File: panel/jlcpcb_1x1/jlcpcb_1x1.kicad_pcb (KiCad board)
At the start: 4 copper layers, 70.5 x 70.5 mm, 185 parts, among them U108 Single Buffer - 74LVC1G125GV,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, U109 3.3v LDO - TLV74133PDBVR

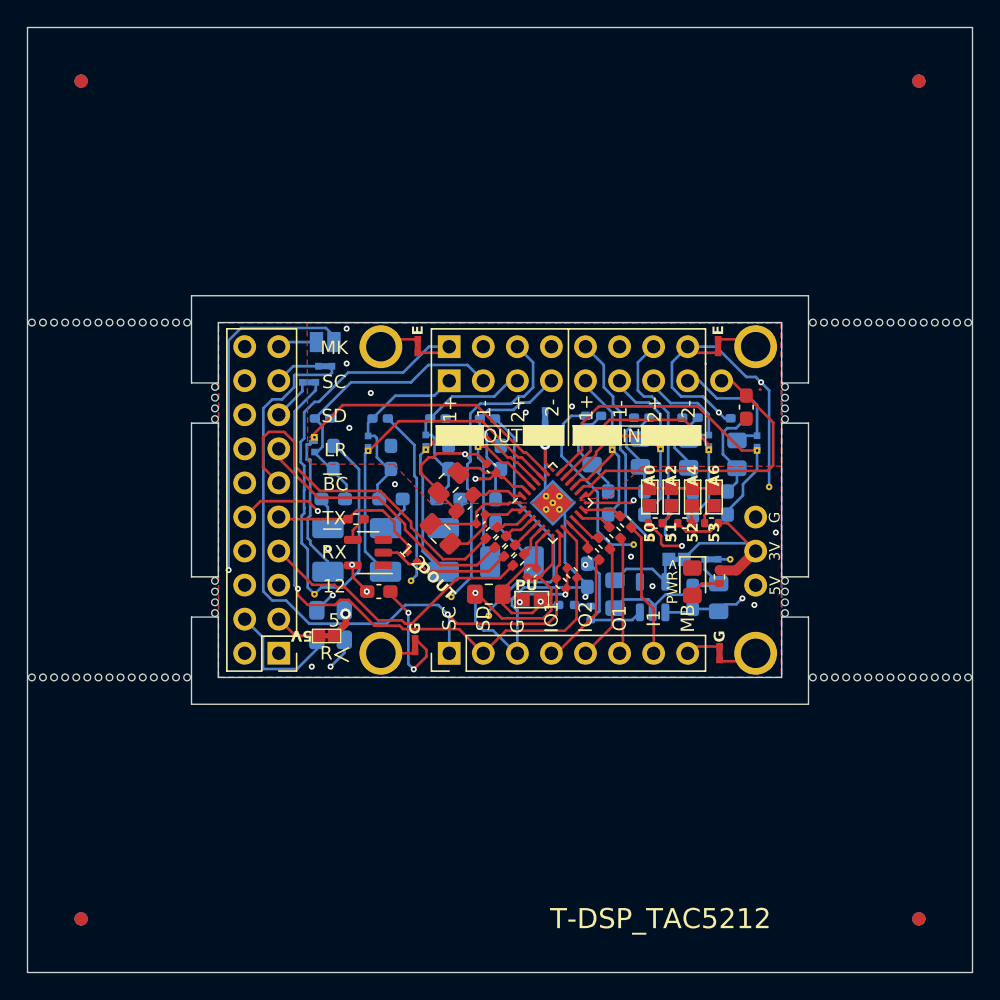
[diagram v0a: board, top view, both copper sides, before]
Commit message: update
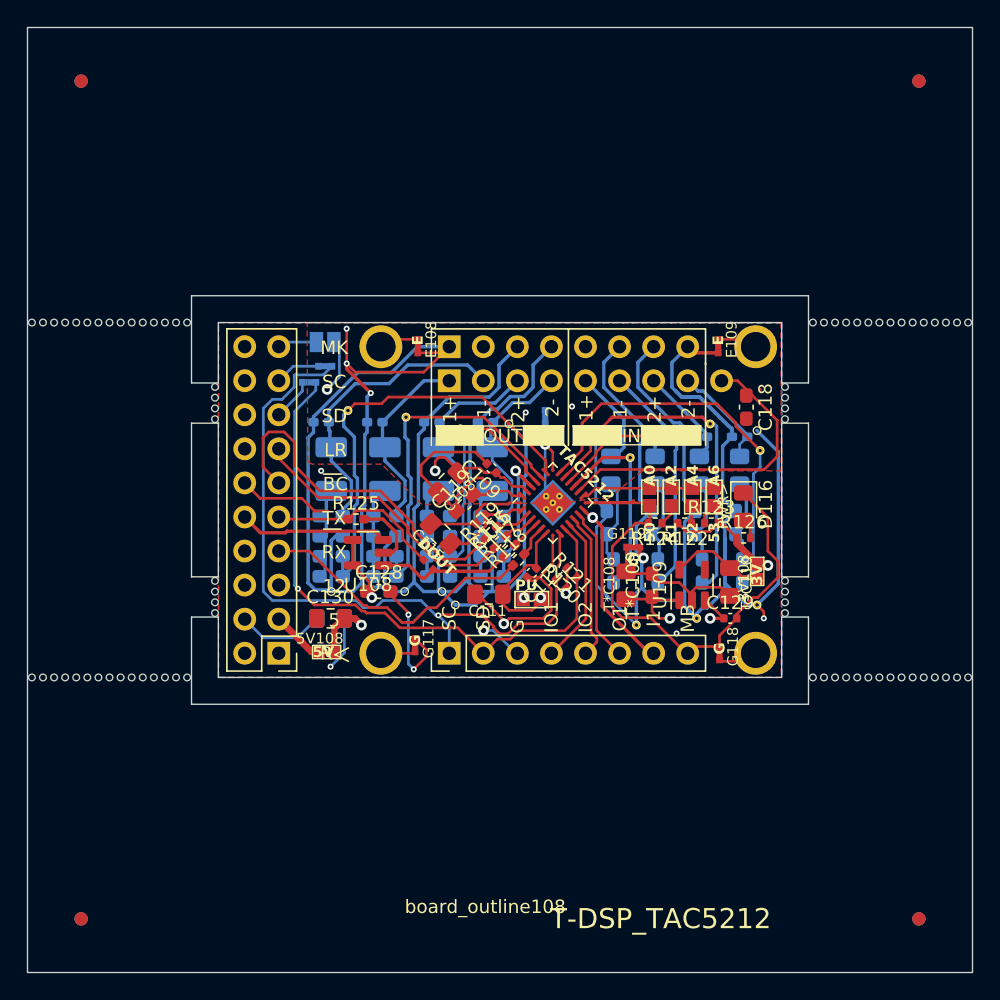
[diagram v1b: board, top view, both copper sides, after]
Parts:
- removed G115: VIA, project_fp:via
- removed OM1: Jump Filter, project_fp:jumper_slice_via_alt_text
- removed OM2, OP1, OP2: Jump Filter, project_fp:jumper_slice_via
- removed R110, R112, R113, R114: 0 Ohm, project_fp:R_0402_1005Metric_Pad0.72x0.64mm_HandSolder
- removed R128: 2.21k ohm, project_fp:R_0402_1005Metric
- removed SCL109: jumper, Resistor_SMD:R_0402_1005Metric_Pad0.72x0.64mm_HandSolder
- added G123: SMD ROUTING PAD, project_fp:SMD_ROUTING_PAD, B.Cu at (149.2, 49.6)
- added OUTM1: VIA, project_fp:via, B.Cu at (137.2, 48.6)
- added OUTP1: VIA, project_fp:via, B.Cu at (141.5, 49.1)
- added OUTP2: VIA, project_fp:via, B.Cu at (145.5, 49.9)
- added R127: DNP, Capacitor_SMD:C_0603_1608Metric_Pad1.08x0.95mm_HandSolder, B.Cu at (139.9, 59.4)
- added R129: 0 ohm, Capacitor_SMD:C_0603_1608Metric_Pad1.08x0.95mm_HandSolder, B.Cu at (139.9, 56.4)
- added R130: 100K, Capacitor_SMD:C_0603_1608Metric_Pad1.08x0.95mm_HandSolder, B.Cu at (166.1, 56.9)
- added R131: DNP, Capacitor_SMD:C_0603_1608Metric_Pad1.08x0.95mm_HandSolder, B.Cu at (143.9, 59.4)
- added R132: 10 ohm, Capacitor_SMD:C_0603_1608Metric_Pad1.08x0.95mm_HandSolder, B.Cu at (143.9, 60.9)
- added R133: 0 ohm, Capacitor_SMD:C_0603_1608Metric_Pad1.08x0.95mm_HandSolder, B.Cu at (143.9, 56.4)
- added R134: DNP, Capacitor_SMD:C_0603_1608Metric_Pad1.08x0.95mm_HandSolder, B.Cu at (147.9, 59.4)
- added R135: 10 ohm, Capacitor_SMD:C_0603_1608Metric_Pad1.08x0.95mm_HandSolder, B.Cu at (147.9, 60.9)
- added R136: 0 ohm, Capacitor_SMD:C_0603_1608Metric_Pad1.08x0.95mm_HandSolder, B.Cu at (147.9, 56.4)
- added R137: 100K, Capacitor_SMD:C_0603_1608Metric_Pad1.08x0.95mm_HandSolder, B.Cu at (163.1, 56.9)
- added R138: 100K, Capacitor_SMD:C_0603_1608Metric_Pad1.08x0.95mm_HandSolder, B.Cu at (159.8, 56.9)
- added R139: 100K, Capacitor_SMD:C_0603_1608Metric_Pad1.08x0.95mm_HandSolder, B.Cu at (156.5, 56.9)
- 3V108, C130, G119, NT108, T*C108, T*C109, T*C110, U109: moved to F.Cu
- C113: value 0.047uF -> 0.0047µF (4.7nF); footprint project_fp:C_0603_1608Metric_Pad1.08x0.95mm_HandSolder -> Capacitor_SMD:C_0603_1608Metric_Pad1.08x0.95mm_HandSolder
- C114, C120, C122: value 47uF -> 0.0047µF (4.7nF); footprint project_fp:CP_EIA-3528-21_Kemet-B_Pad1.50x2.35mm_HandSolder -> Capacitor_SMD:C_0603_1608Metric_Pad1.08x0.95mm_HandSolder
- C117, C121, C123: value 0.047uF -> 47uF; footprint project_fp:C_0603_1608Metric_Pad1.08x0.95mm_HandSolder -> project_fp:CP_EIA-3528-21_Kemet-B_Pad1.50x2.35mm_HandSolder
- C124: value 10UF -> 10UF confirm polarity
- C129: value 1uF -> 0.1uF; footprint project_fp:C_0603_1608Metric_Pad1.08x0.95mm_HandSolder -> project_fp:C_0402_1005Metric; moved to F.Cu
- D108, D109, D110, D111, D112: value TPD1E1B04 - 0402 size -> TPD1E10B06
- G108, G109, G110, G111, G112: footprint project_fp:via -> project_fp:SMD_ROUTING_PAD; moved to B.Cu
- G113, G114, G116: moved to B.Cu
- INM1, INM2, INP1, INP2: value Jump Filter -> VIA; footprint project_fp:jumper_slice_via -> project_fp:via
- R108, R111: value 100 -> 10 ohm; footprint project_fp:R_0603_1608Metric_Pad1.05x0.95mm_HandSolder -> Capacitor_SMD:C_0603_1608Metric_Pad1.08x0.95mm_HandSolder
- R109: value 100 -> DNP; footprint project_fp:R_0603_1608Metric_Pad1.05x0.95mm_HandSolder -> Capacitor_SMD:C_0603_1608Metric_Pad1.08x0.95mm_HandSolder
- R116: value 100 -> 0 ohm; footprint project_fp:R_0603_1608Metric_Pad1.05x0.95mm_HandSolder -> Capacitor_SMD:C_0603_1608Metric_Pad1.08x0.95mm_HandSolder
- R117, R125: value 49.9 ohm -> 27 ohm
- U108: value Single Buffer - 74LVC1G125GV,125 - SOT-23-5 -> Single Buffer with Tri-state Passthru - SN74LVC1G66DCK - SOT-23-5
- board_outline108: footprint project_fp:audio_module_board_outline_50x34.5_d1 -> project_fp:audio_module_board_outline_50x34.5_e1
- moved G112 16.7 mm to (145.2, 63.1), turned to 180 degrees
- moved G110 16.1 mm to (144.2, 62.1), turned to 180 degrees
- moved G113 14.0 mm to (158.7, 64.6), turned to 180 degrees
- moved G108 12.5 mm to (167.7, 50.1), turned to 180 degrees
- moved R116 12.3 mm to (135.9, 56.4), turned to 180 degrees
- moved C129 11.1 mm to (165.7, 64.1), turned to 0 degrees
- moved R111 10.5 mm to (135.9, 60.9)
- moved G116 8.85 mm to (167.7, 63.1), turned to 180 degrees
- moved T*C110 8.62 mm to (165.6, 61.3)
- moved T*C108 6.96 mm to (157.9, 61.6)
- moved D116 6.77 mm to (166.7, 55.6)
- moved G111 6.72 mm to (141.4, 62.1), turned to 180 degrees
- moved 3V108 6.07 mm to (167.7, 60.6), turned to -90 degrees
- moved C110 6.03 mm to (139.9, 52.9)
- moved G109 6.00 mm to (135.9, 62.1), turned to 180 degrees
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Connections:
- C110 pad 1: Board_0-OUT1P -> Board_0-Net-(C110-Pad1)
- C110 pad 2: Board_0-Net-(C110-Pad2) -> Board_0-OUT1P+
- C113 pad 1: Board_0-OUT1P+ -> Board_0-Net-(C110-Pad1)
- C114 pad 1: Board_0-OUT1M -> Board_0-Net-(C114-Pad1)
- C114 pad 2: Board_0-Net-(C114-Pad2) -> Board_0-Earth
- C117 pad 1: Board_0-OUT1M+ -> Board_0-Net-(C114-Pad1)
- C117 pad 2: Board_0-Earth -> Board_0-OUT1M+
- C120 pad 1: Board_0-OUT2P -> Board_0-Net-(C120-Pad1)
- C120 pad 2: Board_0-Net-(C120-Pad2) -> Board_0-Earth
- C121 pad 1: Board_0-OUT2P+ -> Board_0-Net-(C120-Pad1)
- C121 pad 2: Board_0-Earth -> Board_0-OUT2P+
- C122 pad 1: Board_0-OUT2M -> Board_0-Net-(C122-Pad1)
- C122 pad 2: Board_0-Net-(C122-Pad2) -> Board_0-Earth
- C123 pad 1: Board_0-OUT2M+ -> Board_0-Net-(C122-Pad1)
- C123 pad 2: Board_0-Earth -> Board_0-OUT2M+
- D112 pad 1: Board_0-Net-(C124-Pad1) -> Board_0-IN2M+
- D113 pad 1: Board_0-Net-(C125-Pad1) -> Board_0-IN2P+
- D114 pad 1: Board_0-Net-(C126-Pad1) -> Board_0-IN1M+
- D115 pad 1: Board_0-Net-(C127-Pad1) -> Board_0-IN1P+
- INM1 pad 1: Board_0-IN1M+ -> Board_0-IN1M
- INM2 pad 1: Board_0-IN2M+ -> Board_0-IN2M
- INP1 pad 1: Board_0-IN1P+ -> Board_0-IN1P
- INP2 pad 1: Board_0-IN2P+ -> Board_0-IN2P
- R108 pad 1: Board_0-OUT1P+ -> Board_0-Net-(C110-Pad1)
- R108 pad 2: Board_0-Net-(C110-Pad2) -> Board_0-OUT1P
- R109 pad 1: Board_0-OUT1M+ -> Board_0-Net-(C114-Pad1)
- R109 pad 2: Board_0-Net-(C114-Pad2) -> Board_0-OUT1M
- R111 pad 1: Board_0-OUT2P+ -> Board_0-Net-(C114-Pad1)
- R111 pad 2: Board_0-Net-(C120-Pad2) -> Board_0-OUT1M
- R116 pad 1: Board_0-OUT2M+ -> Board_0-OUT1M+
- R116 pad 2: Board_0-Net-(C122-Pad2) -> Board_0-Net-(C114-Pad1)
- R125 pad 2: Board_0-Net-(U108-Y) -> Board_0-Net-(U108-B)
- TAC5212 pad 10: Board_0-Net-(TAC5212-GPIO2) -> Board_0-GPIO2
- TAC5212 pad 11: Board_0-Net-(TAC5212-GPO1) -> Board_0-GPO1
- TAC5212 pad 12: Board_0-Net-(TAC5212-GPI1) -> Board_0-GPI1
- TAC5212 pad 9: Board_0-Net-(TAC5212-GPIO1) -> Board_0-GPIO1
- U108 pad 1: Board_0-GNDD -> Board_0-5212_DOUT1
- U108 pad 2: Board_0-5212_DOUT1 -> Board_0-Net-(U108-B)
- U108 pad 4: Board_0-Net-(U108-Y) -> Board_0-3.3v_IDE
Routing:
- net Board_0-Earth: track 185.5 -> 295.5 mm, vias 11 -> 8
- net Board_0-GPI1: track 71.6 -> 43.5 mm, vias 1 -> 2
- net Board_0-GNDD: track 108.7 -> 135.8 mm, vias 15 -> 7
- net Board_0-IN1M: track 14.1 -> 21.4 mm
- net Board_0-IN2P: track 19.6 -> 26.4 mm
- net Board_0-Net-(C120-Pad1): track 0.00 -> 6.73 mm
- net Board_0-Net-(C110-Pad1): track 0.00 -> 6.73 mm
- net Board_0-Net-(C122-Pad1): track 0.00 -> 6.69 mm
- net Board_0-Net-(C114-Pad1): track 0.00 -> 5.65 mm
- net Board_0-IN1P: track 9.60 -> 14.9 mm
- net Board_0-IN2M: track 25.0 -> 30.2 mm
- net Board_0-Net-(U108-B): track 0.00 -> 5.13 mm
- net Board_0-5V: track 34.4 -> 29.3 mm
- net Board_0-Net-(C122-Pad2): track 4.01 -> 0.00 mm
- net Board_0-3.3V_LDO: track 41.5 -> 38.5 mm, vias 1 -> 2
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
